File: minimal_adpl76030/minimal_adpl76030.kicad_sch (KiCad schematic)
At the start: 49 parts, among them J1 CLP-104-02-G-D-BE, J3 FW-04-03-G-D-085-155, Q1 60 V, Q2 60 V, Q3 25 V, Q4 25 V, U1 ADPL76030EUFD-PBF

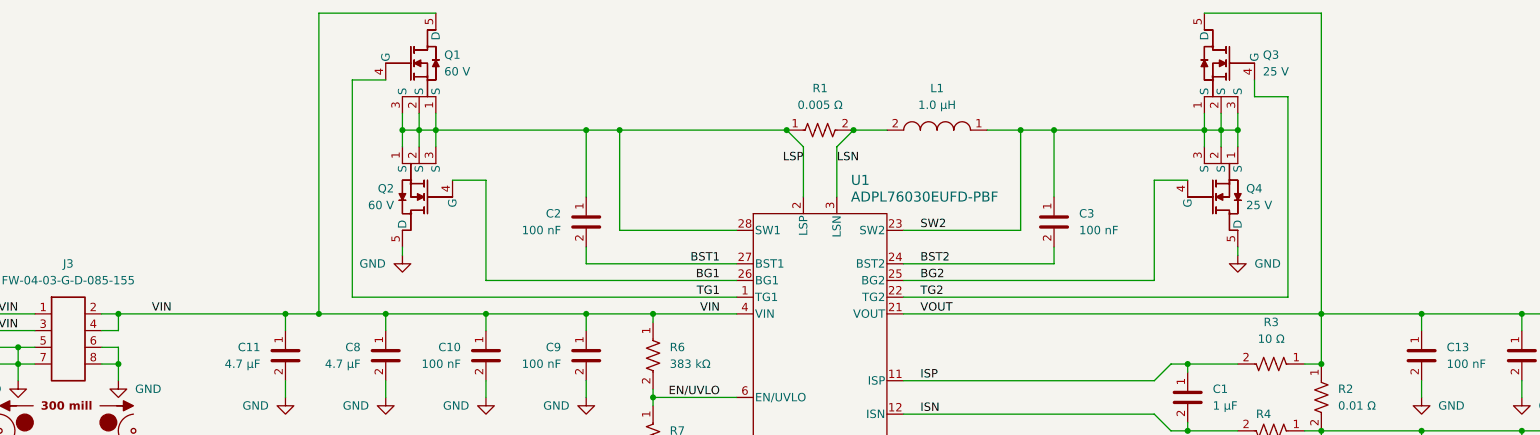
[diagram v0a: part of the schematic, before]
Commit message: backup
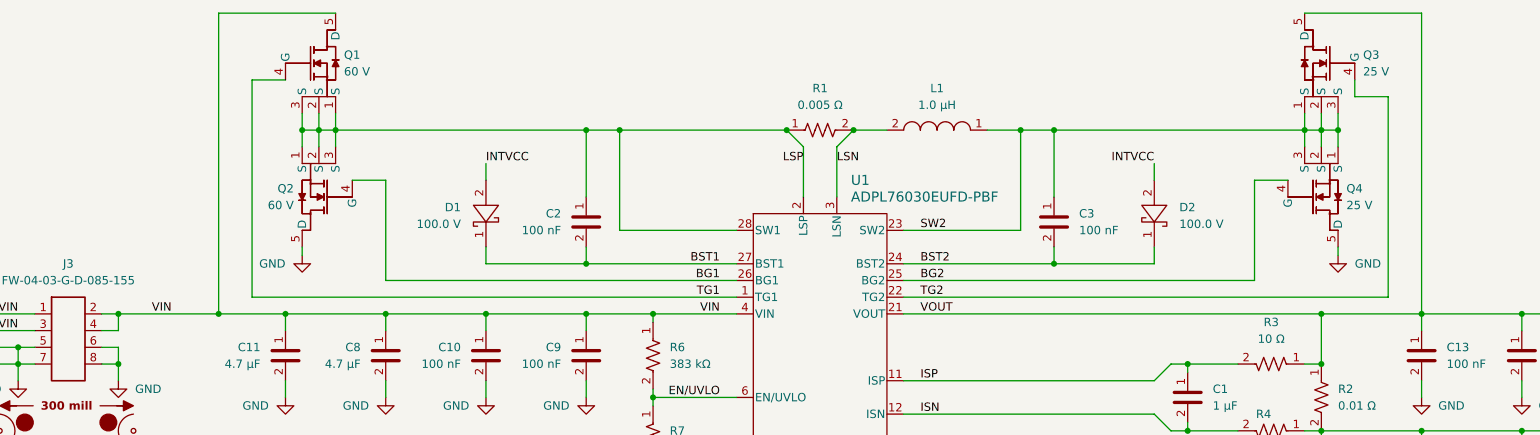
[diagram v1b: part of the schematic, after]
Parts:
- added D1, D2: 100.0 V, diode_footprints:SOD323F, symbol DIODES_BAT46WJ,115_DATA_BASE:D_BAT46WJ,115
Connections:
- net BST1: now also D1.1
- net BST2: now also D2.1
- net INTVCC: now also D1.2, D2.2
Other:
- moved on the sheet: Q1, Q2, Q3, Q4
